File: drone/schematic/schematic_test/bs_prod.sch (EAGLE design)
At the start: 35 parts, among them SW1 418117270902, U1 ATMEGA328P_PDIP, U2 RFM69HW, U3 RFM69HW, Y1 16MHz

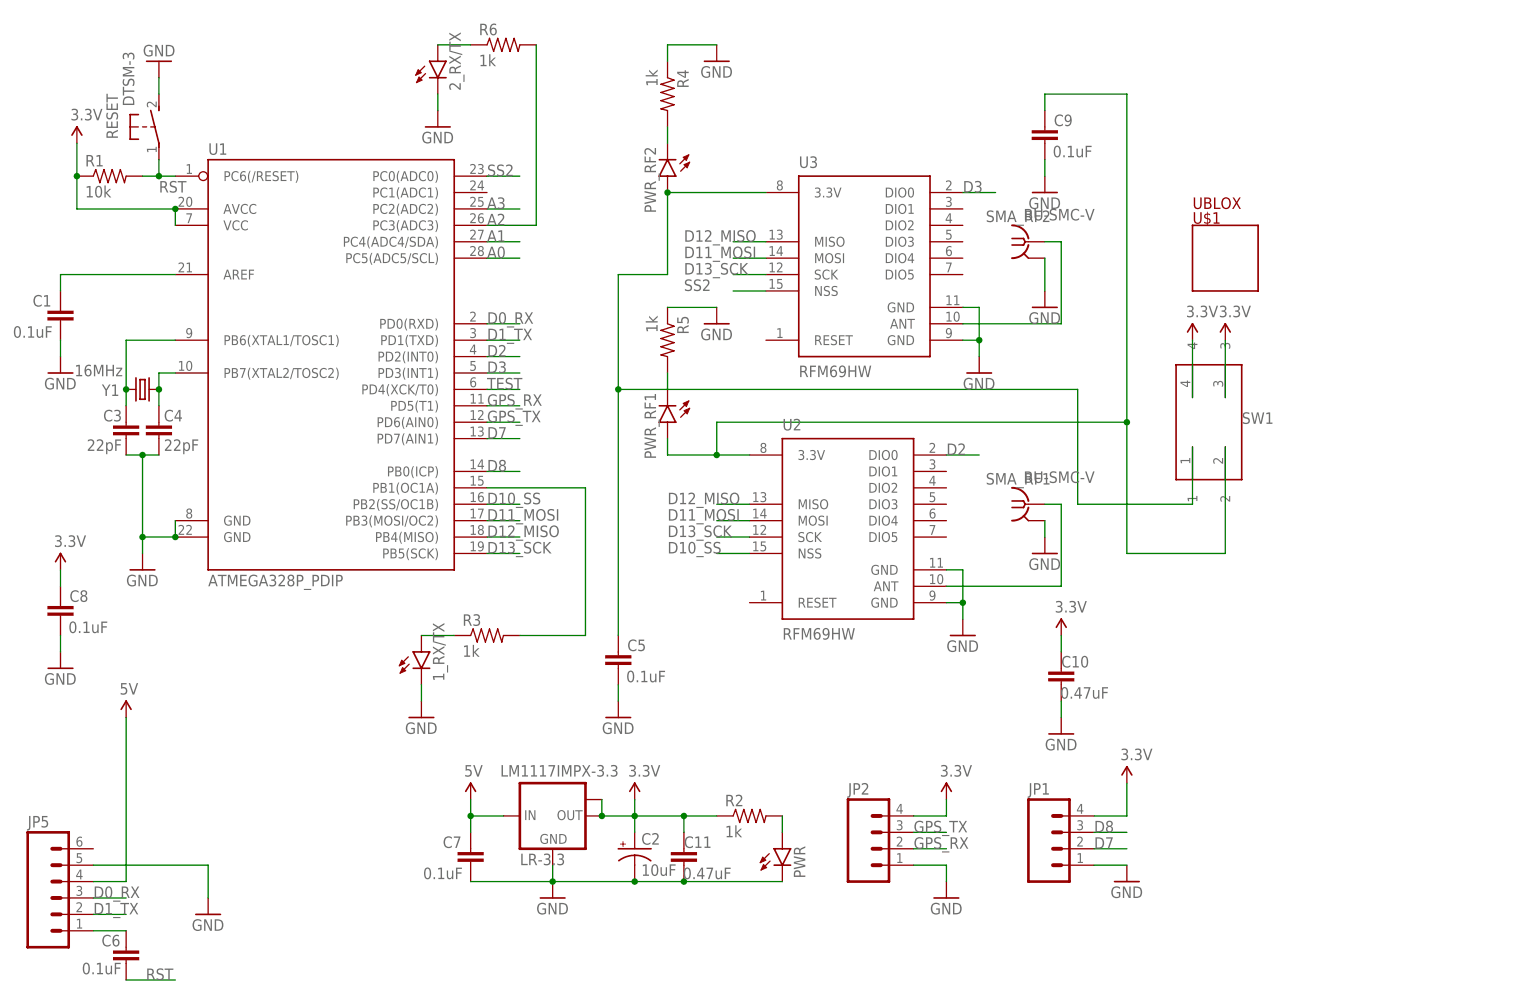
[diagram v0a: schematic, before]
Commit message: current drone schematic
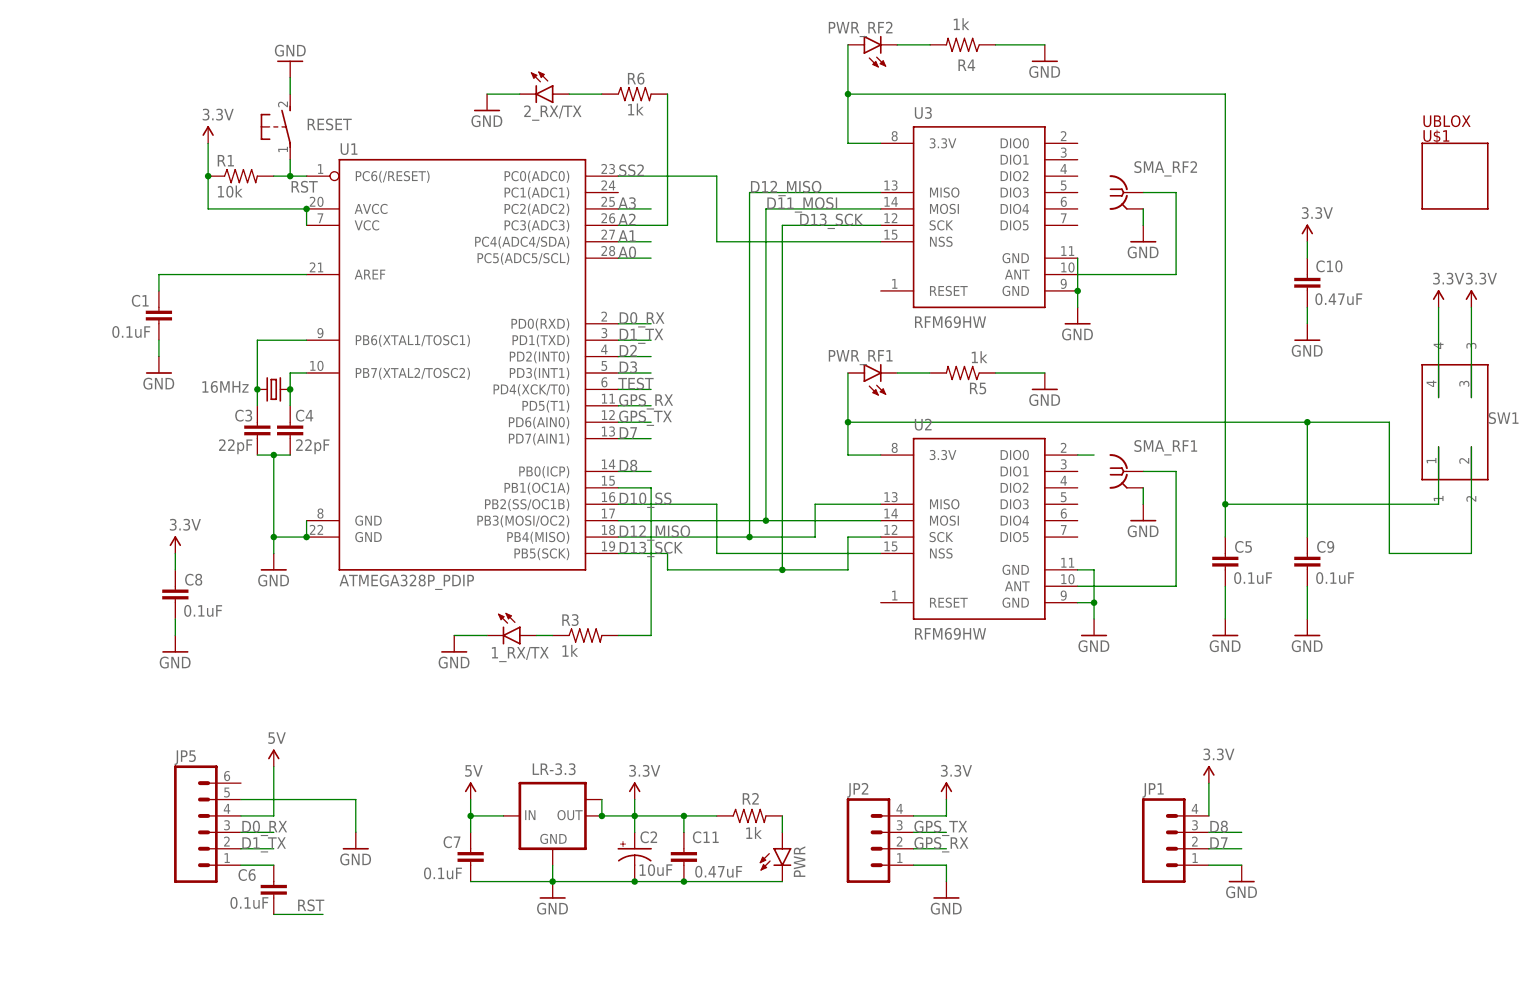
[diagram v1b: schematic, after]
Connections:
- new net N$2: U2.DIO0
- net D2: no longer U2.DIO0
- net D3: no longer U3.DIO0
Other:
- moved on the sheet: 1_RX/TX, 2_RX/TX, C1, C10, C3, C4, C5, C6, C8, C9, JP1, JP5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
